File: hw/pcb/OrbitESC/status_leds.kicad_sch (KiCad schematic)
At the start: 18 parts, among them U12 74HC595, U4 74HC596

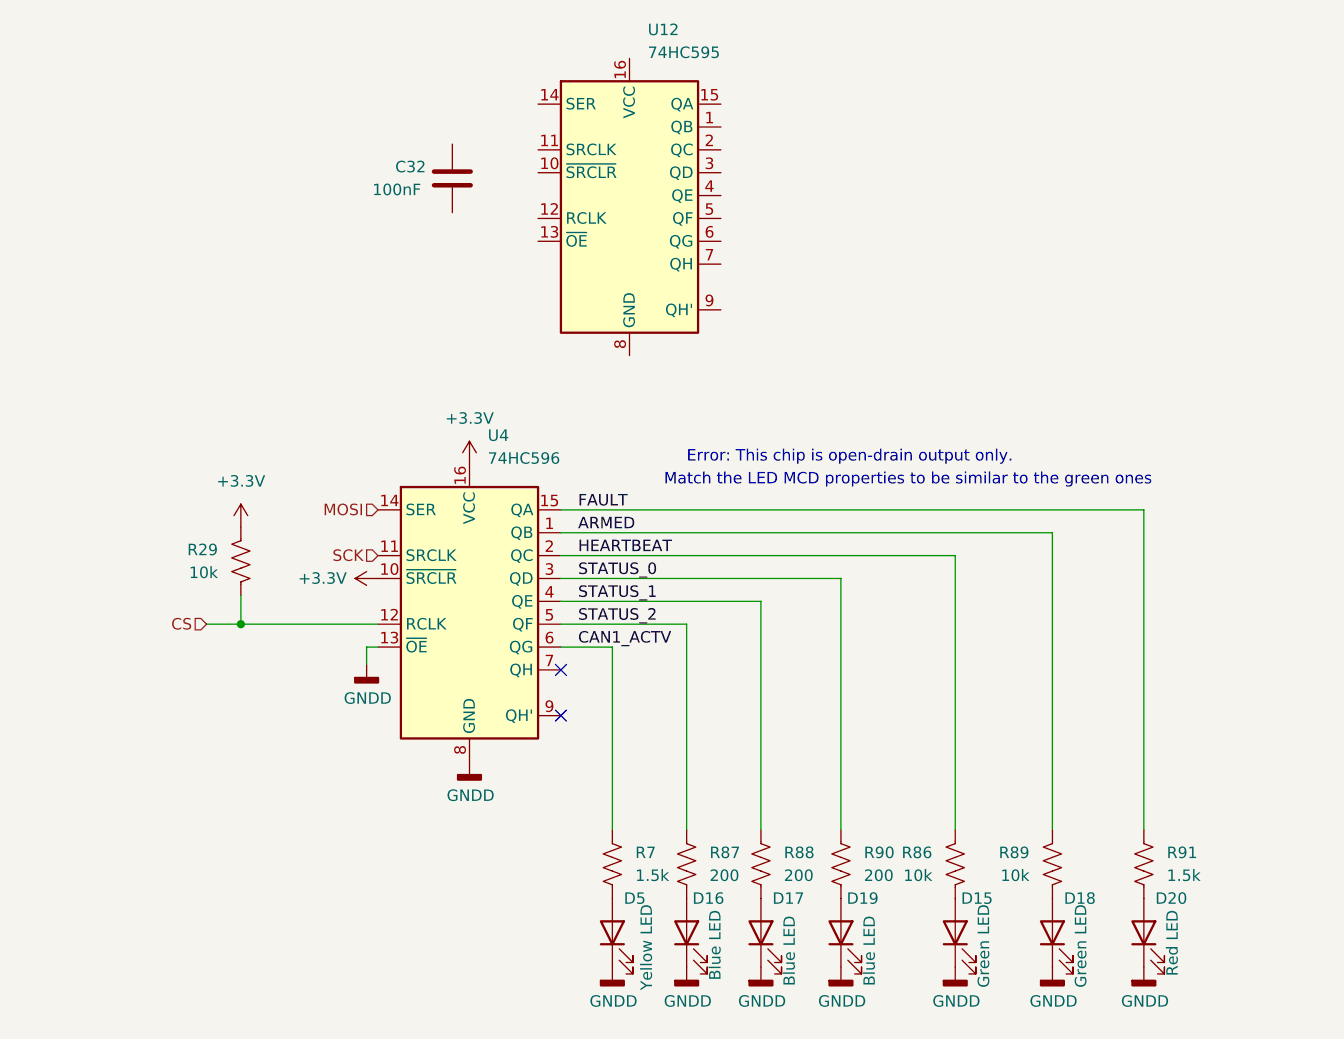
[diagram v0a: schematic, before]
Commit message: Sync lunch schematic update
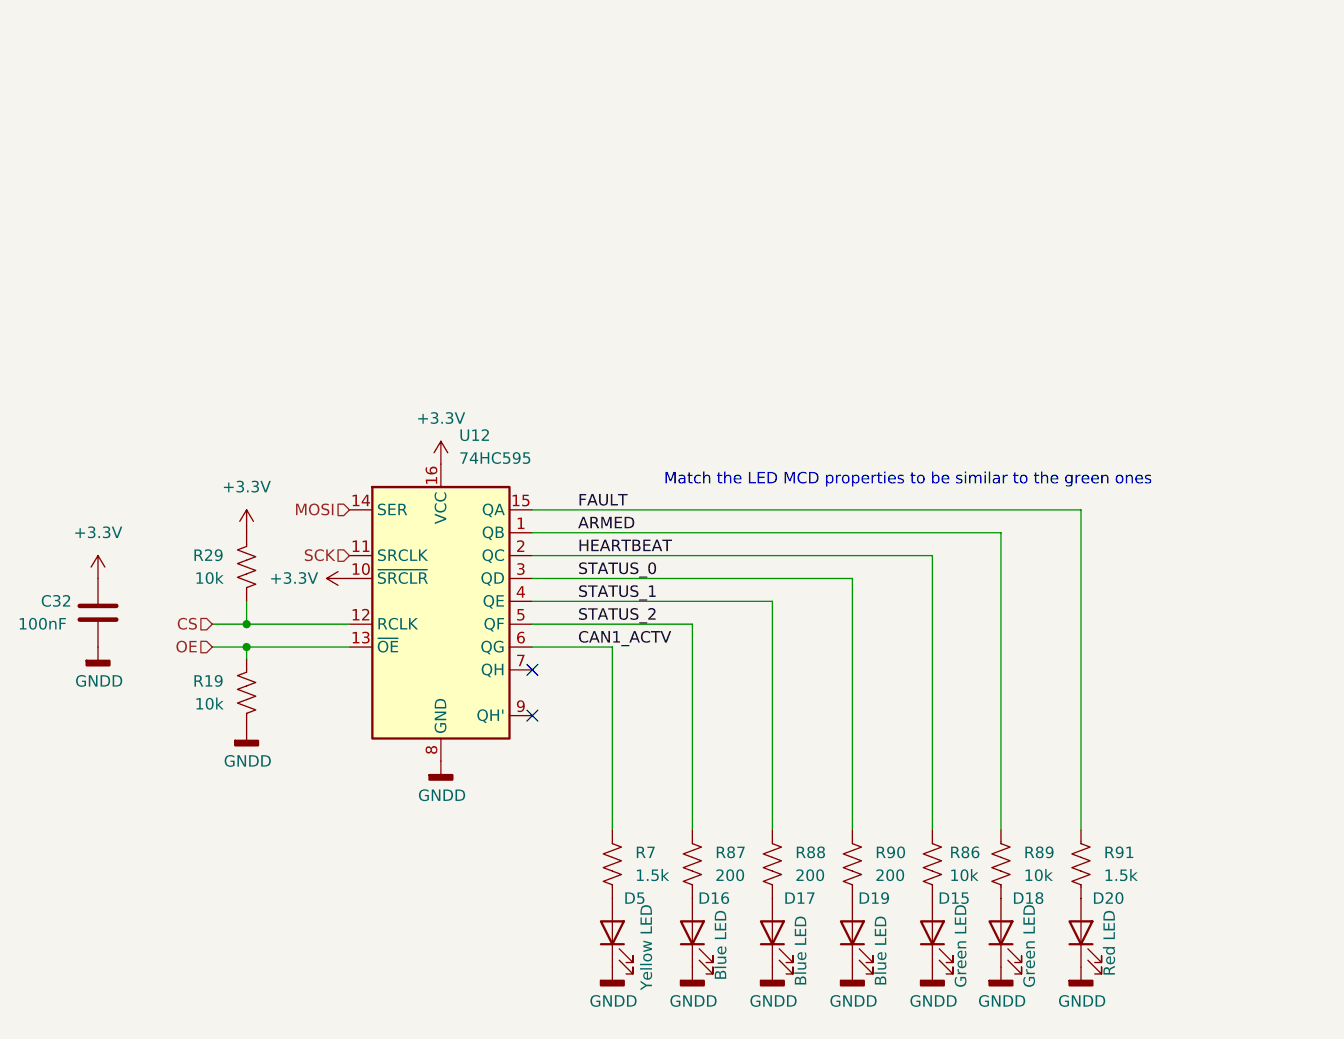
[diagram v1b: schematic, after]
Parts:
- removed U4: 74HC596, Package_SO:TSSOP-16_4.4x5mm_P0.65mm, symbol 74xx:74HC596
- added R19: 10k, Resistor_SMD:R_0402_1005Metric, symbol Device:R_US
- U12: footprint (none) -> Package_SO:SOIC-16_3.9x9.9mm_P1.27mm; JLCPCB (none) -> C5947
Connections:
- net +3.3V: now also C32.2, U12.10 (~{SRCLR}), U12.16 (VCC)
- net ARMED: now also R89.1, U12.1 (QB); no longer R89.2
- net CAN1_ACTV: now also U12.6 (QG)
- net CS: now also U12.12 (RCLK)
- net FAULT: now also U12.15 (QA)
- net GNDD: now also C32.1, U12.8 (GND), R19.1
- net HEARTBEAT: now also R86.1, U12.2 (QC); no longer R86.2
- net MOSI: now also U12.14 (SER)
- net SCK: now also U12.11 (SRCLK)
- net STATUS_0: now also U12.3 (QD)
- net STATUS_1: now also U12.4 (QE)
- net STATUS_2: now also U12.5 (QF)
- net at D15.2 (A): now also R86.2; no longer R86.1
- net at D18.2 (A): now also R89.2; no longer R89.1
- net OE: now reaches U12.13 (~{OE})
- net OE: now also R19.2
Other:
- note removed: "Error: This chip is open-drain output only."
- moved on the sheet: C32, D15, D16, D17, D18, D19, D20, R29, R86, R87, R88, R89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
